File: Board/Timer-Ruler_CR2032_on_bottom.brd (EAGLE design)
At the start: 100 x 80 mm, 33 parts, among them U1 ATMEGA328P_TQFP, Y1 8MHZ

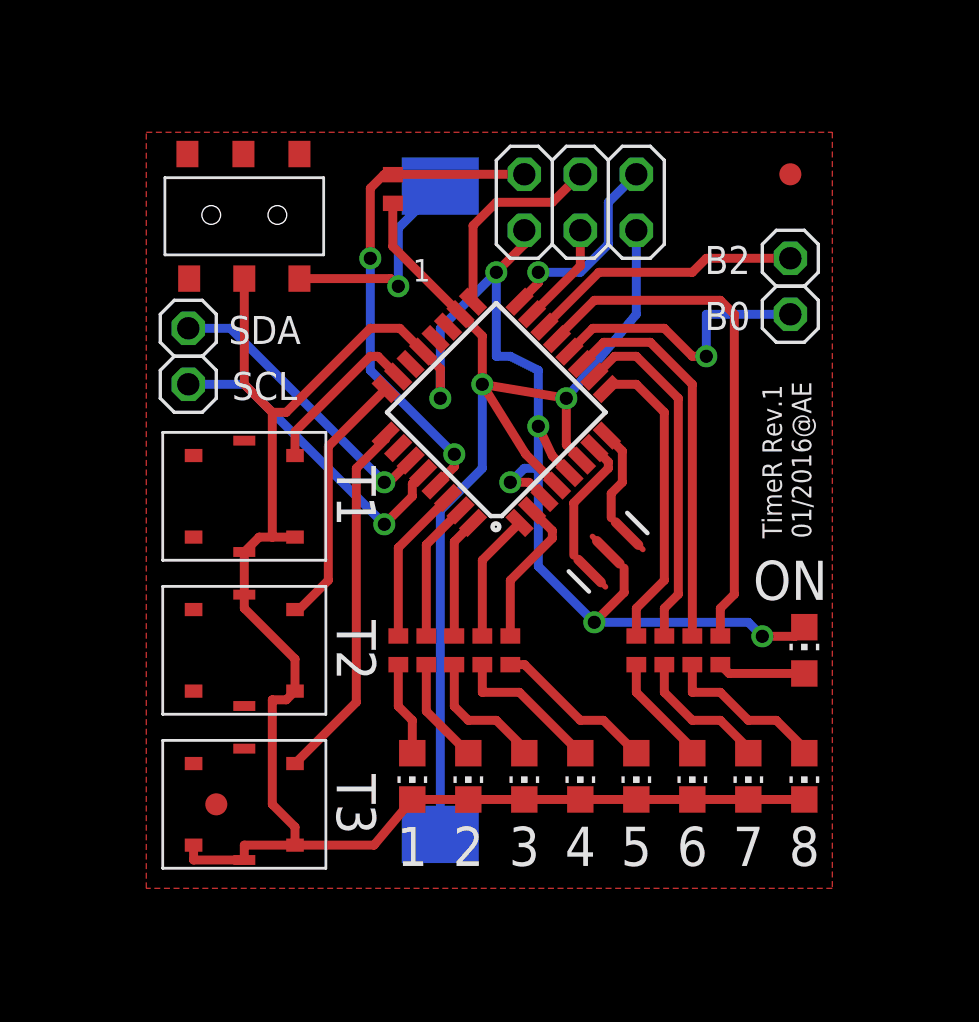
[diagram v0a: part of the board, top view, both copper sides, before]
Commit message: update
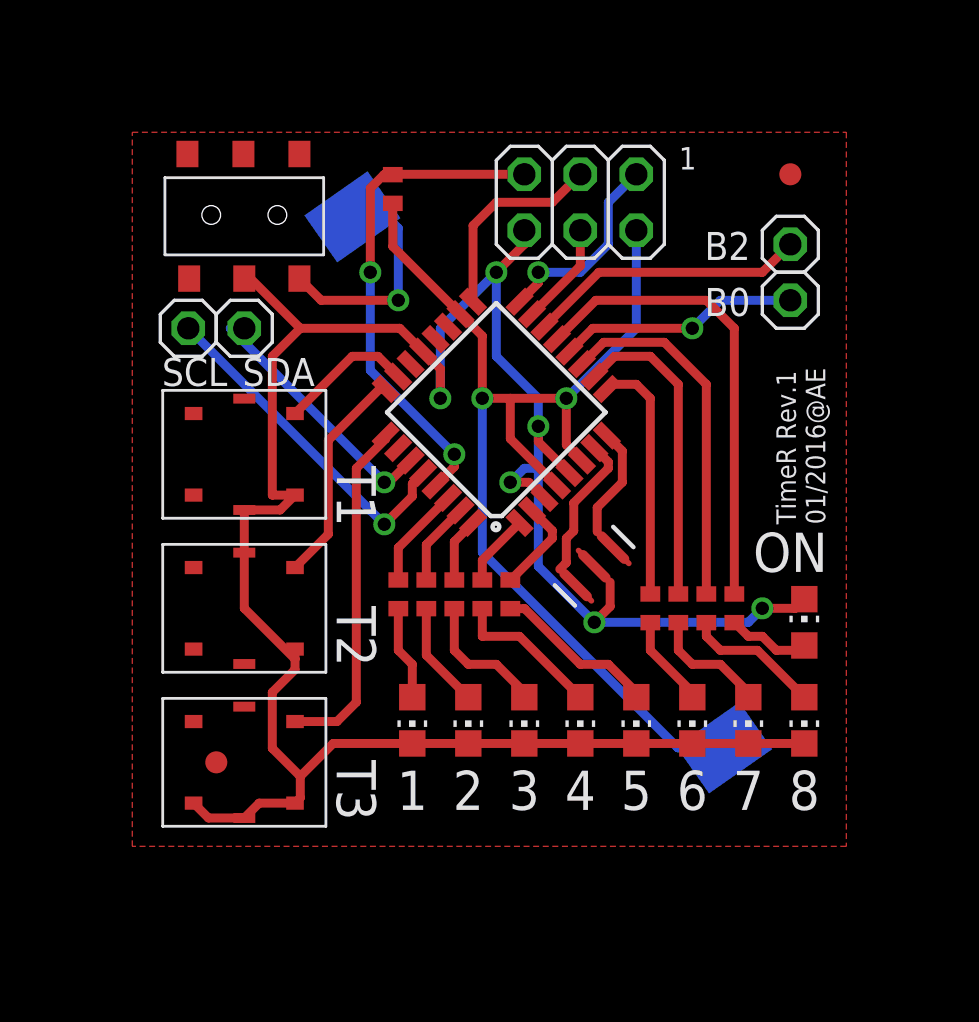
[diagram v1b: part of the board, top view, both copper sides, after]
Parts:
- B0, B2, SCL, SDA: value (none) -> nur PAD, keine Stiftleiste
- JP1: value ISP -> nur PAD, keine Stiftleiste
- moved U$3 4.62 mm to (38.7, 28.6), turned to 55 degrees
- moved R1 2.54 mm to (32.4, 23.5)
- moved R2 2.54 mm to (33.7, 23.5)
- moved R3 2.54 mm to (34.9, 23.5)
- moved R4 2.54 mm to (36.2, 23.5)
- moved R5 2.54 mm to (37.5, 23.5)
- moved LED1 2.54 mm to (33.0, 17.8)
- moved LED2 2.54 mm to (35.6, 17.8)
- moved LED3 2.54 mm to (38.1, 17.8)
- moved LED4 2.54 mm to (40.6, 17.8)
- moved LED5 2.54 mm to (43.2, 17.8)
- moved LED6 2.54 mm to (45.7, 17.8)
- moved LED7 2.54 mm to (48.3, 17.8)
- moved LED8 2.54 mm to (50.8, 17.8)
- moved SCL 2.54 mm to (22.9, 35.6)
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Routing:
- net GND: track 118.1 -> 113.1 mm
- net LED6: track 13.9 -> 11.2 mm
- net LED9: track 23.9 -> 21.3 mm
- net LED2: track 6.34 -> 3.80 mm
- net LED4: track 5.83 -> 3.29 mm
- net LED1: track 7.20 -> 4.66 mm
- net LED3: track 5.48 -> 2.94 mm
- net LED5: track 6.87 -> 4.36 mm
- net PB0: track 12.9 -> 11.0 mm
- net TASTER2: track 11.8 -> 9.96 mm
- net LED7: track 16.0 -> 14.2 mm
- net TASTER1: track 7.56 -> 6.14 mm
- net N$8: track 7.61 -> 6.21 mm
- net SDA: track 13.4 -> 12.1 mm
- net LED8: track 17.6 -> 16.3 mm
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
